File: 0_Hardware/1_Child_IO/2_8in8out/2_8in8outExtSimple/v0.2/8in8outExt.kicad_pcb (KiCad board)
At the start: 2 copper layers, 101.6 x 42 mm, 73 parts, among them P1 CONN_10X2, Q1 PNP, Q10 NPN, Q11 NPN, Q12 NPN, Q13 NPN, Q14 NPN, Q15 NPN, Q16 NPN, Q19 NPN, Q2 PNP, Q3 PNP, Q4 PNP, Q5 PNP, Q6 PNP, Q7 PNP, Q8 PNP, Q9 NPN, SW1 SKQGAKE010

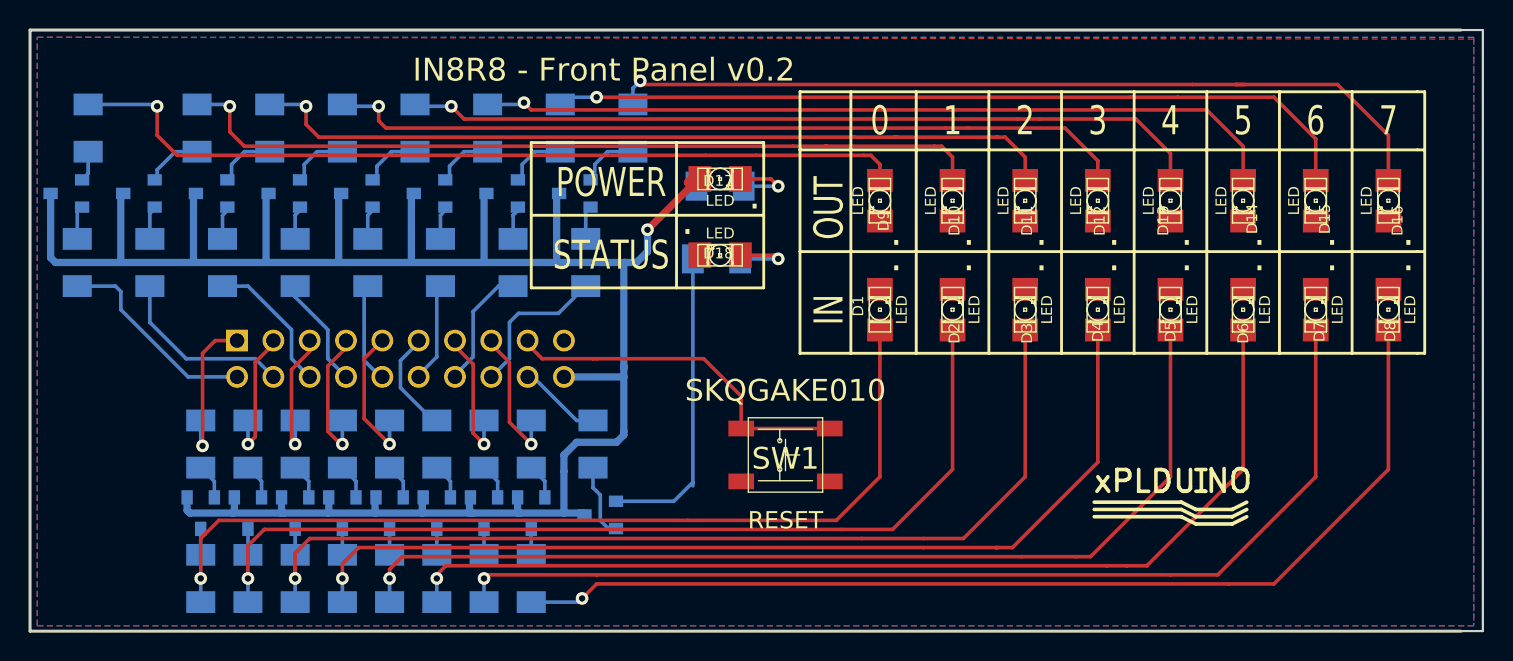
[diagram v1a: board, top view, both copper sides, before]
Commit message: Revert "skilkscreen + gerber"
This reverts commit f66d5581d9f6963949e67885314110cfecfc1ca6.
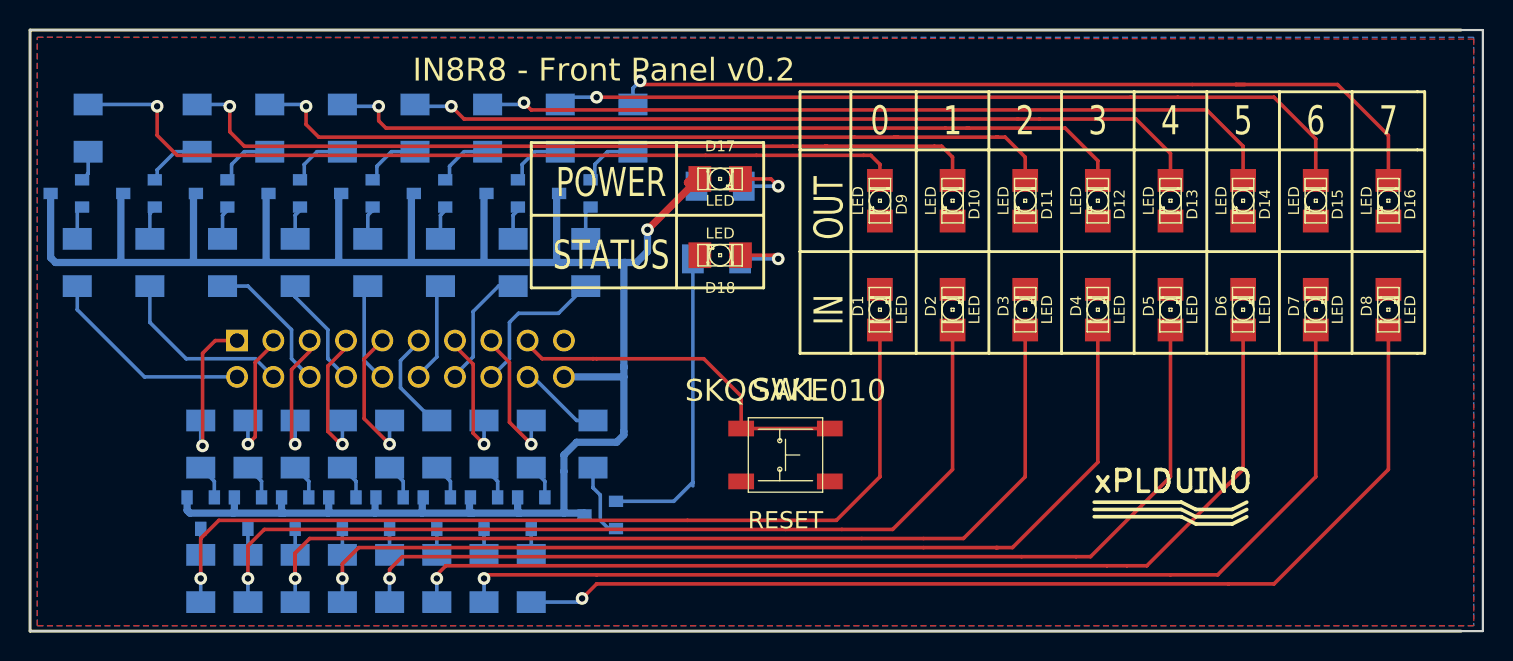
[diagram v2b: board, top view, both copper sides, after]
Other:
- board text removed: "."
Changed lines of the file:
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@@
     (area 76.964334 69.045001 188.035001 116.3345)
     (thickness 1.6)
-    (drawings 79)
-    (tracks 403)
+    (drawings 61)
+    (tracks 401)
     (zones 0)
     (modules 73)
@@
     (18 B.Paste user)
     (19 F.Paste user)
-    (20 B.SilkS user)
+    (20 B.SilkS user hide)
     (21 F.SilkS user)
     (22 B.Mask user)
@@
       (plotothertext true)
       (plotinvisibletext false)
-      (padsonsilk true)
+      (padsonsilk false)
       (subtractmaskfromsilk false)
       (outputformat 1)
@@
   (module SKQGAKE010 (layer F.Cu)
     (at 139.192 103.632 180)
-    (fp_text reference SW1 (at 0 -0.254 180) (layer F.SilkS)
+    (fp_text reference SW1 (at 0 4.572 180) (layer F.SilkS)
       (effects (font (size 1.524 1.524) (thickness 0.3048)))
     )
@@
     (tags "LED1206 SMD")
     (attr smd)
-    (fp_text reference D7 (at -1.524 0.254 90) (layer F.SilkS)
+    (fp_text reference D7 (at 0.254 -1.524 90) (layer F.SilkS)
       (effects (font (size 0.762 0.762) (thickness 0.0889)))
     )
@@
     (tags "LED1206 SMD")
     (attr smd)
-    (fp_text reference D2 (at -1.651 0.127 90) (layer F.SilkS)
+    (fp_text reference D2 (at 0.254 -1.524 90) (layer F.SilkS)
       (effects (font (size 0.762 0.762) (thickness 0.0889)))
     )
@@
     (tags "LED1206 SMD")
     (attr smd)
-    (fp_text reference D18 (at 0.127 0.127 180) (layer F.SilkS)
+    (fp_text reference D18 (at 0 -2.286 180) (layer F.SilkS)
       (effects (font (size 0.762 0.762) (thickness 0.0889)))
     )
@@
     (tags "LED1206 SMD")
     (attr smd)
-    (fp_text reference D3 (at -1.651 0.127 90) (layer F.SilkS)
+    (fp_text reference D3 (at 0.254 -1.524 90) (layer F.SilkS)
       (effects (font (size 0.762 0.762) (thickness 0.0889)))
     )
@@
     (tags "LED1206 SMD")
     (attr smd)
-    (fp_text reference D17 (at -0.127 0.127) (layer F.SilkS)
+    (fp_text reference D17 (at 0 -2.286) (layer F.SilkS)
       (effects (font (size 0.762 0.762) (thickness 0.0889)))
     )
@@
     (tags "LED1206 SMD")
     (attr smd)
-    (fp_text reference D4 (at -1.524 0 90) (layer F.SilkS)
+    (fp_text reference D4 (at 0.254 -1.524 90) (layer F.SilkS)
       (effects (font (size 0.762 0.762) (thickness 0.0889)))
     )
@@
     (tags "LED1206 SMD")
     (attr smd)
-    (fp_text reference D5 (at -1.524 0 90) (layer F.SilkS)
+    (fp_text reference D5 (at 0.254 -1.524 90) (layer F.SilkS)
       (effects (font (size 0.762 0.762) (thickness 0.0889)))
     )
@@
     (tags "LED1206 SMD")
     (attr smd)
-    (fp_text reference D6 (at -1.651 0 90) (layer F.SilkS)
+    (fp_text reference D6 (at 0.254 -1.524 90) (layer F.SilkS)
       (effects (font (size 0.762 0.762) (thickness 0.0889)))
     )
@@
     (tags "LED1206 SMD")
     (attr smd)
-    (fp_text reference D12 (at 1.397 -0.127 270) (layer F.SilkS)
+    (fp_text reference D12 (at 0.254 -1.524 270) (layer F.SilkS)
       (effects (font (size 0.762 0.762) (thickness 0.0889)))
     )
@@
     (tags "LED1206 SMD")
     (attr smd)
-    (fp_text reference D8 (at -1.524 0.127 90) (layer F.SilkS)
+    (fp_text reference D8 (at 0.254 -1.524 90) (layer F.SilkS)
       (effects (font (size 0.762 0.762) (thickness 0.0889)))
     )
@@
     (tags "LED1206 SMD")
     (attr smd)
-    (fp_text reference D9 (at 1.397 -0.254 270) (layer F.SilkS)
+    (fp_text reference D9 (at 0.254 -1.524 270) (layer F.SilkS)
       (effects (font (size 0.762 0.762) (thickness 0.0889)))
     )
@@
     (tags "LED1206 SMD")
     (attr smd)
-    (fp_text reference D10 (at 1.397 -0.127 270) (layer F.SilkS)
+    (fp_text reference D10 (at 0.254 -1.524 270) (layer F.SilkS)
       (effects (font (size 0.762 0.762) (thickness 0.0889)))
     )
@@
     (tags "LED1206 SMD")
     (attr smd)
-    (fp_text reference D11 (at 1.397 -0.127 270) (layer F.SilkS)
+    (fp_text reference D11 (at 0.254 -1.524 270) (layer F.SilkS)
       (effects (font (size 0.762 0.762) (thickness 0.0889)))
     )
@@
     (tags "LED1206 SMD")
     (attr smd)
-    (fp_text reference D16 (at 1.397 -0.635 270) (layer F.SilkS)
+    (fp_text reference D16 (at 0.254 -1.524 270) (layer F.SilkS)
       (effects (font (size 0.762 0.762) (thickness 0.0889)))
     )
@@
     (tags "LED1206 SMD")
     (attr smd)
-    (fp_text reference D15 (at 1.27 -0.635 270) (layer F.SilkS)
+    (fp_text reference D15 (at 0.254 -1.524 270) (layer F.SilkS)
       (effects (font (size 0.762 0.762) (thickness 0.0889)))
     )
@@
     (tags "LED1206 SMD")
     (attr smd)
-    (fp_text reference D14 (at 1.27 -0.635 270) (layer F.SilkS)
+    (fp_text reference D14 (at 0.254 -1.524 270) (layer F.SilkS)
       (effects (font (size 0.762 0.762) (thickness 0.0889)))
     )
@@
     (tags "LED1206 SMD")
     (attr smd)
-    (fp_text reference D13 (at 1.397 0.508 270) (layer F.SilkS)
+    (fp_text reference D13 (at 0.254 -1.524 270) (layer F.SilkS)
       (effects (font (size 0.762 0.762) (thickness 0.0889)))
     )
@@
     )
   )
-  (gr_line (start 111.252 92.964) (end 113.284 92.964) (angle 90) (layer B.SilkS) (width 0.2))
-  (gr_text . (at 146.939 89.789) (layer F.SilkS)
-    (effects (font (size 2 2) (thickness 0.25)))
-  )
-  (gr_text . (at 146.939 88.011) (layer F.SilkS)
-    (effects (font (size 2 2) (thickness 0.25)))
-  )
-  (gr_text . (at 152.019 88.011) (layer F.SilkS)
-    (effects (font (size 2 2) (thickness 0.25)))
-  )
-  (gr_text . (at 152.019 89.789) (layer F.SilkS)
-    (effects (font (size 2 2) (thickness 0.25)))
-  )
-  (gr_text . (at 157.099 89.789) (layer F.SilkS)
-    (effects (font (size 2 2) (thickness 0.25)))
-  )
-  (gr_text . (at 157.099 88.011) (layer F.SilkS)
-    (effects (font (size 2 2) (thickness 0.25)))
-  )
-  (gr_text . (at 162.179 88.011) (layer F.SilkS)
-    (effects (font (size 2 2) (thickness 0.25)))
-  )
-  (gr_text . (at 162.179 89.789) (layer F.SilkS)
-    (effects (font (size 2 2) (thickness 0.25)))
-  )
-  (gr_text . (at 167.259 89.789) (layer F.SilkS)
-    (effects (font (size 2 2) (thickness 0.25)))
-  )
-  (gr_text . (at 172.339 89.789) (layer F.SilkS)
-    (effects (font (size 2 2) (thickness 0.25)))
-  )
-  (gr_text . (at 177.419 89.789) (layer F.SilkS)
-    (effects (font (size 2 2) (thickness 0.25)))
-  )
-  (gr_text . (at 167.259 88.011) (layer F.SilkS)
-    (effects (font (size 2 2) (thickness 0.25)))
-  )
-  (gr_text . (at 172.339 88.011) (layer F.SilkS)
-    (effects (font (size 2 2) (thickness 0.25)))
-  )
-  (gr_text . (at 177.419 88.011) (layer F.SilkS)
-    (effects (font (size 2 2) (thickness 0.25)))
-  )
-  (gr_text . (at 132.334 87.249) (layer F.SilkS)
-    (effects (font (size 2 2) (thickness 0.25)))
-  )
-  (gr_text . (at 137.033 85.471) (layer F.SilkS)
-    (effects (font (size 2 2) (thickness 0.25)))
-  )
-  (gr_text . (at 182.753 88.011) (layer F.SilkS)
-    (effects (font (size 2 2) (thickness 0.25)))
-  )
-  (gr_text . (at 182.753 89.789) (layer F.SilkS)
-    (effects (font (size 2 2) (thickness 0.25)))
-  )
   (gr_line (start 183.388 82.296) (end 183.896 82.296) (angle 90) (layer F.SilkS) (width 0.2))
   (gr_line (start 183.388 89.408) (end 183.896 89.408) (angle 90) (layer F.SilkS) (width 0.2))
@@
   )
   (gr_line (start 181.356 93.472) (end 181.356 83.82) (angle 90) (layer Cmts.User) (width 0.2))
+  (gr_line (start 111.252 92.964) (end 113.284 92.964) (angle 90) (layer F.Mask) (width 0.2))
   (gr_line (start 187.96 73.914) (end 187.96 115.951) (angle 90) (layer Edge.Cuts) (width 0.15))
   (gr_line (start 186.436 73.914) (end 187.96 73.914) (angle 90) (layer Edge.Cuts) (width 0.15))
@@
   (segment (start 110.617 83.439) (end 111.633 82.423) (width 0.254) (layer B.Cu) (net 63))
   (segment (start 111.633 82.423) (end 113.284 82.423) (width 0.254) (layer B.Cu) (net 63))
-  (segment (start 89.662 91.821) (end 92.329 91.821) (width 0.254) (layer B.Cu) (net 64))
-  (segment (start 92.71 93.472) (end 97.409 98.171) (width 0.254) (layer B.Cu) (net 64))
-  (segment (start 92.71 92.202) (end 92.71 93.472) (width 0.254) (layer B.Cu) (net 64))
-  (segment (start 92.329 91.821) (end 92.71 92.202) (width 0.254) (layer B.Cu) (net 64))
-  (segment (start 97.409 98.171) (end 100.838 98.171) (width 0.254) (layer B.Cu) (net 64))
+  (segment (start 94.361 98.171) (end 100.838 98.171) (width 0.254) (layer B.Cu) (net 64))
+  (segment (start 89.662 91.821) (end 89.662 93.472) (width 0.254) (layer B.Cu) (net 64))
+  (segment (start 89.662 93.472) (end 94.361 98.171) (width 0.254) (layer B.Cu) (net 64))
   (segment (start 102.108 96.901) (end 103.378 98.171) (width 0.254) (layer B.Cu) (net 65))
   (segment (start 97.282 96.901) (end 102.108 96.901) (width 0.254) (layer B.Cu) (net 65))
